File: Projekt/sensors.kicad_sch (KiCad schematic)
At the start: 11 parts, among them J1 Conn_01x02, U1 LM393

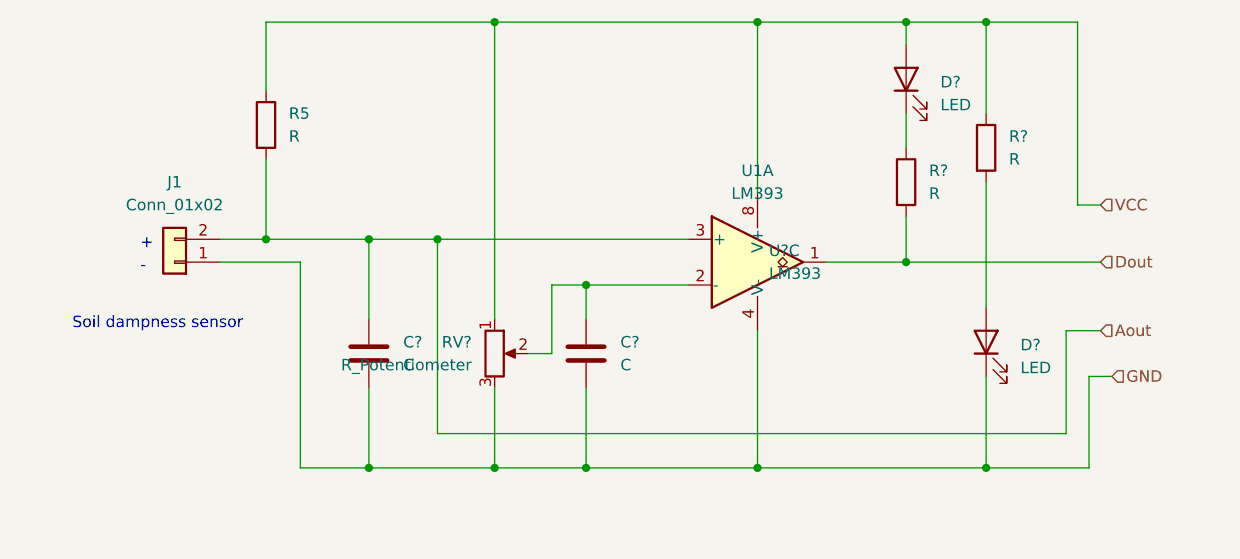
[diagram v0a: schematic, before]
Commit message: Add files via upload
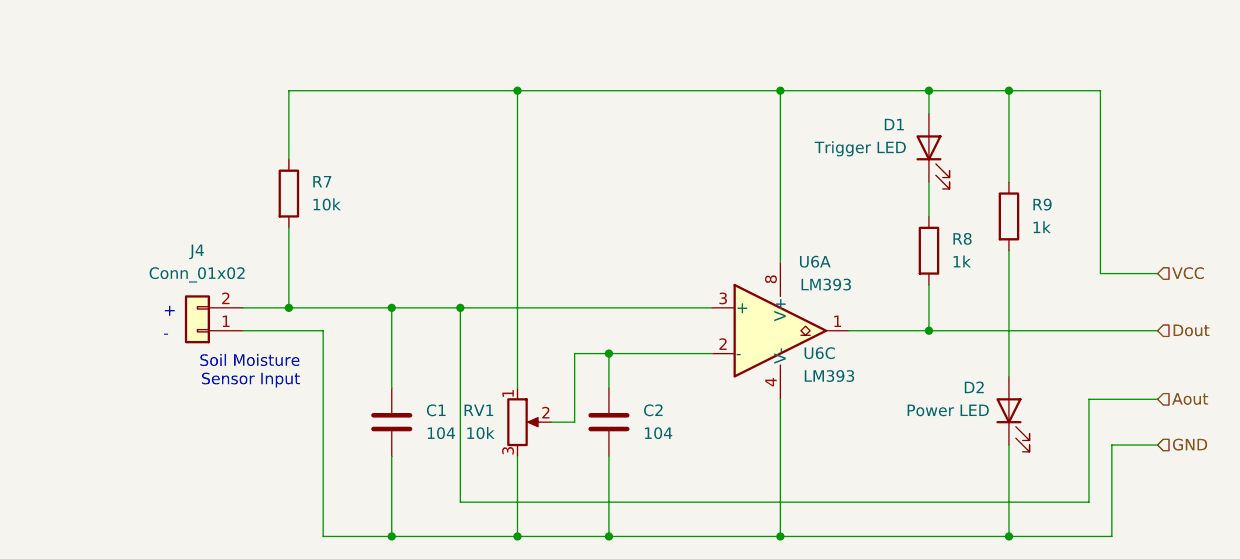
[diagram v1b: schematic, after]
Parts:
- removed C? (x2): C, symbol Device:C
- removed D? (x2): LED, symbol Device:LED
- removed J1: Conn_01x02, symbol Connector_Generic:Conn_01x02
- removed R5, R? (x2): R, symbol Device:R
- removed RV?: R_Potentiometer, symbol Device:R_Potentiometer
- removed U1, U?: LM393, symbol Comparator:LM393
- added C1, C2: 104, symbol Device:C
- added D1: Trigger LED, symbol Device:LED
- added D2: Power LED, symbol Device:LED
- added J4: Conn_01x02, symbol Connector_Generic:Conn_01x02
- added R7: 10k, symbol Device:R
- added R8, R9: 1k, symbol Device:R
- added RV1: 10k, symbol Device:R_Potentiometer
- added U6: LM393, symbol Comparator:LM393
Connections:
- net Aout: now also C1.1, J4.2 (Pin_2), R7.2, U6.3 (+)
- net Dout: now also R8.2, U6.1
- net GND: now also C1.2, C2.2, D2.1 (K), J4.1 (Pin_1), RV1.3, U6.4 (V-)
- net VCC: now also D1.2 (A), R7.1, R9.1, RV1.1, U6.8 (V+)
- new net: D1.1 (K), R8.1
- new net: C2.1, RV1.2, U6.2 (-)
- new net: D2.2 (A), R9.2
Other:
- note added: "Soil Moisture Sensor Input"
- note removed: "Soil dampness sensor"
